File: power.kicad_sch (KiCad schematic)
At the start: 12 parts, among them U4 MIC2288, U6 XC9140

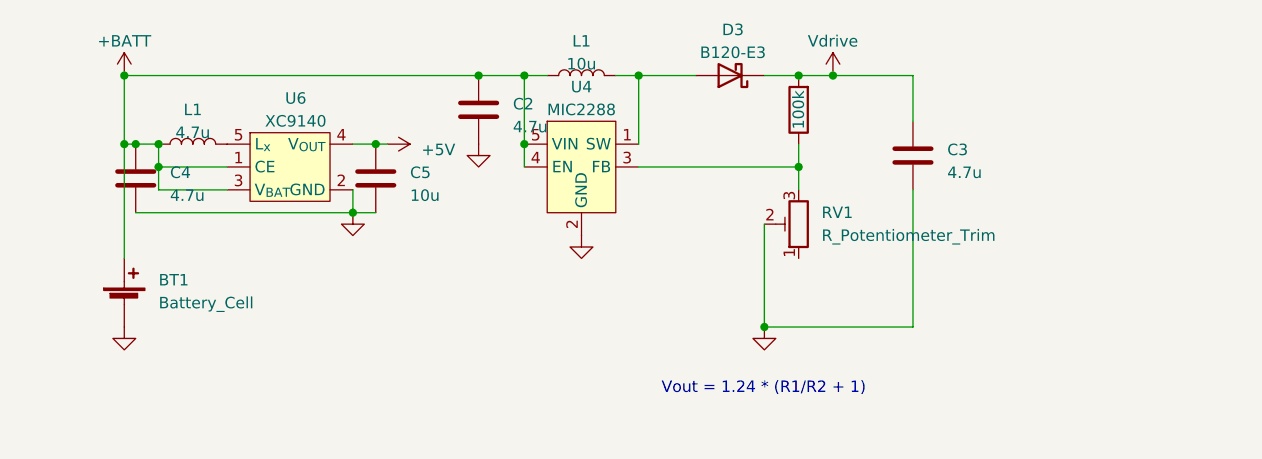
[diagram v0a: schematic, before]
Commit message: Seems reasonable
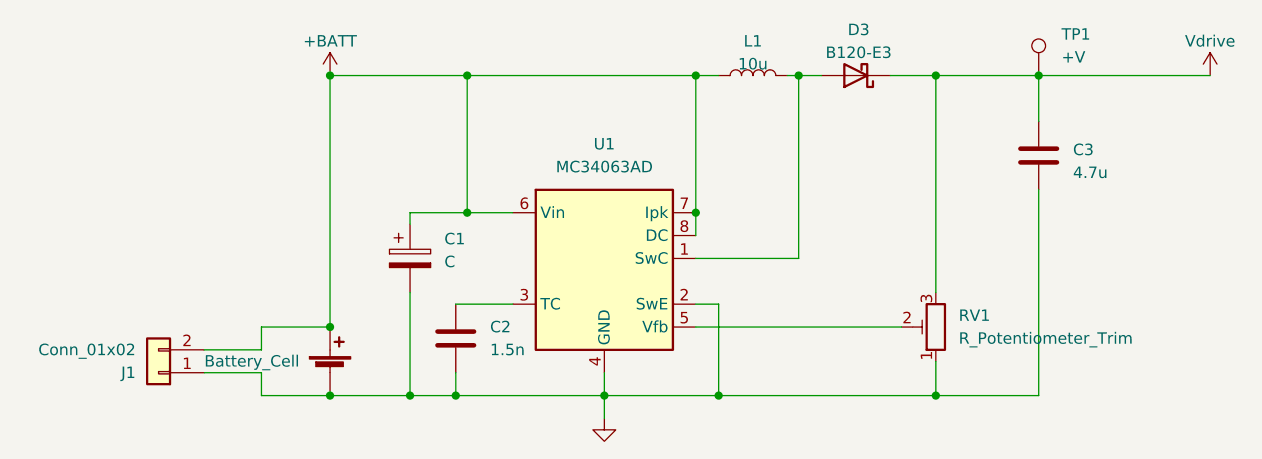
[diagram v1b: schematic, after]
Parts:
- removed C4: 4.7u, Capacitor_SMD:C_1206_3216Metric_Pad1.33x1.80mm_HandSolder, symbol Device:C
- removed C5: 10u, Capacitor_SMD:C_1206_3216Metric_Pad1.33x1.80mm_HandSolder, symbol Device:C
- removed L1: 4.7u, Inductor_SMD:L_Coilcraft_XAL4030-XXX, symbol Device:L
- removed R17: 100k, Resistor_SMD:R_1206_3216Metric_Pad1.30x1.75mm_HandSolder, symbol Device:R
- removed U4: MIC2288, Package_TO_SOT_SMD:SOT-23-5_HandSoldering, symbol custom_symbols:MIC2288
- removed U6: XC9140, Package_SO:TSOP-5_1.65x3.05mm_P0.95mm, symbol custom_symbols:XC9140
- added C1: C, Capacitor_SMD:C_0603_1608Metric, symbol Device:C_Polarized
- added J1: Conn_01x02, Connector_PinHeader_2.54mm:PinHeader_1x02_P2.54mm_Horizontal, symbol Connector_Generic:Conn_01x02
- added TP1: +V, TestPoint:TestPoint_Pad_D1.0mm, symbol Connector:TestPoint
- added U1: MC34063AD, Package_SO:SOIC-8_3.9x4.9mm_P1.27mm, symbol Regulator_Switching:MC34063AD
- C2: value 4.7u -> 1.5n; footprint Capacitor_SMD:C_1206_3216Metric_Pad1.33x1.80mm_HandSolder -> Capacitor_SMD:C_0603_1608Metric
- C3: footprint Capacitor_SMD:C_1206_3216Metric_Pad1.33x1.80mm_HandSolder -> Capacitor_SMD:C_0603_1608Metric
- L1: footprint Inductor_SMD:L_Coilcraft_XAL4030-XXX -> Inductor_SMD:L_1008_2520Metric
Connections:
- net +BATT: now also C1.1, J1.2 (Pin_2), U1.6 (Vin), U1.7 (Ipk), U1.8 (DC); no longer C2.1
- net GND: now also RV1.1, C1.2, J1.1 (Pin_1), U1.2 (SwE), U1.4 (GND); no longer RV1.2
- net Vdrive: now also RV1.3, TP1.1
- net at D3.2 (A), L1.2: now also U1.1 (SwC)
- new net: C2.1, U1.3 (TC)
- new net: RV1.2, U1.5 (Vfb)
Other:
- note removed: "Vout = 1.24 * (R1/R2 + 1)"
- moved on the sheet: C2, C3, D3, L1, RV1
